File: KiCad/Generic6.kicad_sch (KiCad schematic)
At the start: 19 parts, among them J1 Shelly, J2 SPOX, J3 Conn_01x05, U1 ESP32-PICO-MINI-02, U2 LMR16006+FB

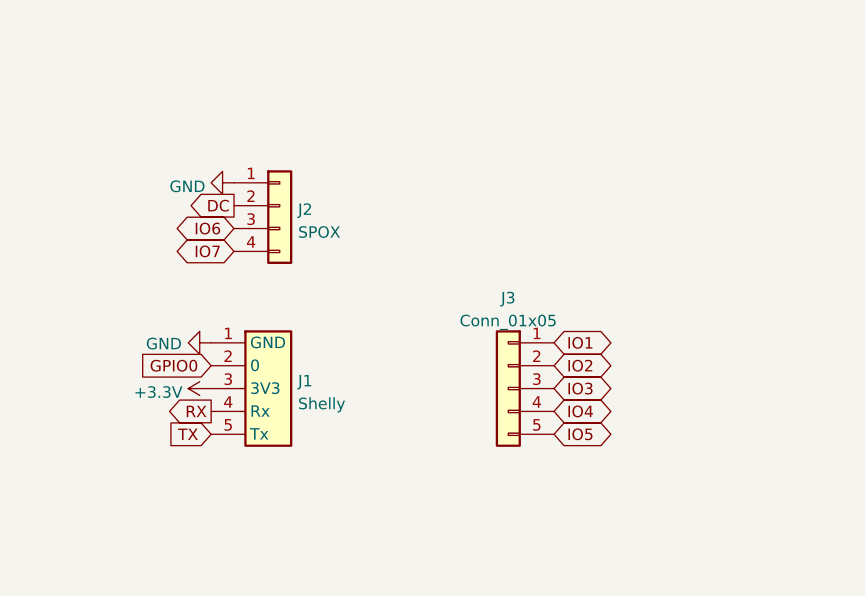
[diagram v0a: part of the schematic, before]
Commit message: Tidy Generic 4 Started on Generic 6
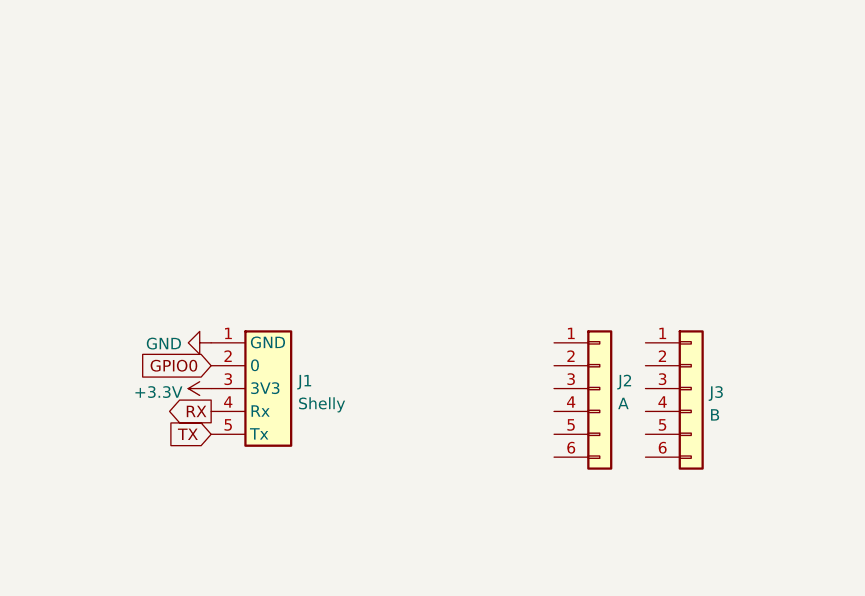
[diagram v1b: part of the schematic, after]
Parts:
- removed J2: SPOX, RevK:Molex_MiniSPOX_H4RA, symbol Connector_Generic:Conn_01x04
- removed J3: Conn_01x05, Connector_PinSocket_2.54mm:PinSocket_1x05_P2.54mm_Vertical, symbol Connector_Generic:Conn_01x05
- added J2: A, Connector_PinHeader_2.54mm:PinHeader_1x05_P2.54mm_Vertical, symbol Connector_Generic:Conn_01x06
- added J3: B, Connector_PinHeader_2.54mm:PinHeader_1x05_P2.54mm_Vertical, symbol Connector_Generic:Conn_01x06
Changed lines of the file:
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@@
     (stroke (width 0) (type default) (color 0 0 0 0))
-  )
-  (global_label "IO4" (shape bidirectional) (at 177.8 106.68 0) (fields_autoplaced)
-    (effects (font (size 1.27 1.27)) (justify left))
-    (property "Intersheet References" "${INTERSHEET_REFS}" (id 0) (at 183.269 106.7594 0)
-      (effects (font (size 1.27 1.27)) (justify left) hide)
-    )
   )
   (global_label "DC" (shape input) (at 136.525 36.83 180) (fields_autoplaced)
@@
     )
   )
-  (global_label "IO2" (shape bidirectional) (at 177.8 101.6 0) (fields_autoplaced)
-    (effects (font (size 1.27 1.27)) (justify left))
-    (property "Intersheet References" "${INTERSHEET_REFS}" (id 0) (at 183.269 101.6794 0)
-      (effects (font (size 1.27 1.27)) (justify left) hide)
-    )
-  )
   (global_label "IO4" (shape bidirectional) (at 50.8 83.82 180) (fields_autoplaced)
     (effects (font (size 1.27 1.27)) (justify right))
@@
     )
   )
-  (global_label "IO3" (shape bidirectional) (at 177.8 104.14 0) (fields_autoplaced)
-    (effects (font (size 1.27 1.27)) (justify left))
-    (property "Intersheet References" "${INTERSHEET_REFS}" (id 0) (at 183.269 104.2194 0)
-      (effects (font (size 1.27 1.27)) (justify left) hide)
-    )
-  )
   (global_label "R" (shape input) (at 81.28 71.12 0) (fields_autoplaced)
     (effects (font (size 1.27 1.27)) (justify left))
     (property "Intersheet References" "${INTERSHEET_REFS}" (id 0) (at 184.15 166.37 0)
       (effects (font (size 1.27 1.27)) hide)
-    )
-  )
-  (global_label "IO5" (shape bidirectional) (at 177.8 109.22 0) (fields_autoplaced)
-    (effects (font (size 1.27 1.27)) (justify left))
-    (property "Intersheet References" "${INTERSHEET_REFS}" (id 0) (at 183.269 109.1406 0)
-      (effects (font (size 1.27 1.27)) (justify left) hide)
     )
   )
@@
     )
   )
-  (global_label "IO7" (shape bidirectional) (at 142.24 88.9 180) (fields_autoplaced)
-    (effects (font (size 1.27 1.27)) (justify right))
-    (property "Intersheet References" "${INTERSHEET_REFS}" (id 0) (at 136.771 88.8206 0)
-      (effects (font (size 1.27 1.27)) (justify right) hide)
-    )
-  )
   (global_label "IO2" (shape bidirectional) (at 81.28 76.2 0) (fields_autoplaced)
     (effects (font (size 1.27 1.27)) (justify left))
@@
     )
   )
-  (global_label "IO6" (shape bidirectional) (at 142.24 86.36 180) (fields_autoplaced)
-    (effects (font (size 1.27 1.27)) (justify right))
-    (property "Intersheet References" "${INTERSHEET_REFS}" (id 0) (at 136.771 86.4394 0)
-      (effects (font (size 1.27 1.27)) (justify right) hide)
-    )
-  )
-  (global_label "DC" (shape output) (at 142.24 83.82 180) (fields_autoplaced)
-    (effects (font (size 1.27 1.27)) (justify right))
-    (property "Intersheet References" "${INTERSHEET_REFS}" (id 0) (at 137.3758 83.7406 0)
-      (effects (font (size 1.27 1.27)) (justify right) hide)
-    )
-  )
-  (global_label "IO1" (shape bidirectional) (at 177.8 99.06 0) (fields_autoplaced)
-    (effects (font (size 1.27 1.27)) (justify left))
-    (property "Intersheet References" "${INTERSHEET_REFS}" (id 0) (at 183.269 99.1394 0)
-      (effects (font (size 1.27 1.27)) (justify left) hide)
-    )
-  )
   (global_label "G" (shape input) (at 53.34 116.84 180) (fields_autoplaced)
     (effects (font (size 1.27 1.27)) (justify right))
@@
     (pin "2")
   )
-  (symbol (lib_id "power:GND") (at 142.24 81.28 270) (unit 1)
-    (in_bom yes) (on_board yes) (fields_autoplaced)
-    (property "Reference" "#PWR09" (id 0) (at 135.89 81.28 0)
-      (effects (font (size 1.27 1.27)) hide)
-    )
-    (property "Value" "GND" (id 1) (at 139.0651 81.7138 90)
-      (effects (font (size 1.27 1.27)) (justify right))
-    )
-    (property "Footprint" "" (id 2) (at 142.24 81.28 0)
-      (effects (font (size 1.27 1.27)) hide)
-    )
-    (property "Datasheet" "" (id 3) (at 142.24 81.28 0)
-      (effects (font (size 1.27 1.27)) hide)
-    )
-    (pin "1")
+  (symbol (lib_id "Connector_Generic:Conn_01x06") (at 193.04 104.14 0) (unit 1)
+    (in_bom yes) (on_board yes) (fields_autoplaced)
+    (property "Reference" "J3" (id 0) (at 195.072 104.5753 0)
+      (effects (font (size 1.27 1.27)) (justify left))
+    )
+    (property "Value" "B" (id 1) (at 195.072 107.1122 0)
+      (effects (font (size 1.27 1.27)) (justify left))
+    )
+    (property "Footprint" "Connector_PinHeader_2.54mm:PinHeader_1x05_P2.54mm_Vertical" (id 2) (at 193.04 104.14 0)
+      (effects (font (size 1.27 1.27)) hide)
+    )
+    (property "Datasheet" "~" (id 3) (at 193.04 104.14 0)
+      (effects (font (size 1.27 1.27)) hide)
+    )
+    (pin "1")
+    (pin "2")
+    (pin "3")
+    (pin "4")
+    (pin "5")
+    (pin "6")
   )
   (symbol (lib_id "Device:R") (at 64.77 27.94 270) (unit 1)
@@
   (symbol (lib_id "power:GND") (at 147.32 53.34 0) (unit 1)
     (in_bom yes) (on_board yes) (fields_autoplaced)
-    (property "Reference" "#PWR010" (id 0) (at 147.32 59.69 0)
+    (property "Reference" "#PWR09" (id 0) (at 147.32 59.69 0)
       (effects (font (size 1.27 1.27)) hide)
     )
@@
     )
     (pin "1")
-  )
-  (symbol (lib_id "Connector_Generic:Conn_01x05") (at 172.72 104.14 0) (mirror y) (unit 1)
-    (in_bom yes) (on_board yes) (fields_autoplaced)
-    (property "Reference" "J3" (id 0) (at 172.72 94.0902 0))
-    (property "Value" "Conn_01x05" (id 1) (at 172.72 96.6271 0))
-    (property "Footprint" "Connector_PinSocket_2.54mm:PinSocket_1x05_P2.54mm_Vertical" (id 2) (at 172.72 104.14 0)
-      (effects (font (size 1.27 1.27)) hide)
-    )
-    (property "Datasheet" "~" (id 3) (at 172.72 104.14 0)
-      (effects (font (size 1.27 1.27)) hide)
-    )
-    (pin "1")
-    (pin "2")
-    (pin "3")
-    (pin "4")
-    (pin "5")
   )
   (symbol (lib_id "RevK:Shelly") (at 144.78 104.14 0) (unit 1)
@@
     (pin "1")
   )
+  (symbol (lib_id "Connector_Generic:Conn_01x06") (at 182.88 104.14 0) (unit 1)
+    (in_bom yes) (on_board yes) (fields_autoplaced)
+    (property "Reference" "J2" (id 0) (at 184.912 103.3053 0)
+      (effects (font (size 1.27 1.27)) (justify left))
+    )
+    (property "Value" "A" (id 1) (at 184.912 105.8422 0)
+      (effects (font (size 1.27 1.27)) (justify left))
+    )
+    (property "Footprint" "Connector_PinHeader_2.54mm:PinHeader_1x05_P2.54mm_Vertical" (id 2) (at 182.88 104.14 0)
+      (effects (font (size 1.27 1.27)) hide)
+    )
+    (property "Datasheet" "~" (id 3) (at 182.88 104.14 0)
+      (effects (font (size 1.27 1.27)) hide)
+    )
+    (pin "1")
+    (pin "2")
+    (pin "3")
+    (pin "4")
+    (pin "5")
+    (pin "6")
+  )
   (symbol (lib_id "Device:C") (at 39.37 27.94 90) (unit 1)
     (in_bom yes) (on_board yes) (fields_autoplaced)
@@
     (pin "2")
   )
-  (symbol (lib_id "Connector_Generic:Conn_01x04") (at 147.32 83.82 0) (unit 1)
-    (in_bom yes) (on_board yes) (fields_autoplaced)
-    (property "Reference" "J2" (id 0) (at 149.352 84.2553 0)
-      (effects (font (size 1.27 1.27)) (justify left))
-    )
-    (property "Value" "SPOX" (id 1) (at 149.352 86.7922 0)
-      (effects (font (size 1.27 1.27)) (justify left))
-    )
-    (property "Footprint" "RevK:Molex_MiniSPOX_H4RA" (id 2) (at 148.59 91.44 0)
-      (effects (font (size 1.27 1.27)) hide)
-    )
-    (property "Datasheet" "~" (id 3) (at 147.32 83.82 0)
-      (effects (font (size 1.27 1.27)) hide)
-    )
-    (pin "1")
-    (pin "2")
-    (pin "3")
-    (pin "4")
-  )
   (symbol (lib_id "power:+3.3V") (at 200.66 38.1 0) (unit 1)
     (in_bom yes) (on_board yes) (fields_autoplaced)
-    (property "Reference" "#PWR011" (id 0) (at 200.66 41.91 0)
+    (property "Reference" "#PWR010" (id 0) (at 200.66 41.91 0)
       (effects (font (size 1.27 1.27)) hide)
     )
@@
   (symbol (lib_id "power:GND") (at 200.66 45.72 0) (unit 1)
     (in_bom yes) (on_board yes) (fields_autoplaced)
-    (property "Reference" "#PWR012" (id 0) (at 200.66 52.07 0)
+    (property "Reference" "#PWR011" (id 0) (at 200.66 52.07 0)
       (effects (font (size 1.27 1.27)) hide)
     )
@@
       (reference "#PWR08") (unit 1) (value "+3.3V") (footprint "")
     )
-    (path "/1e8ea742-99a3-47cc-bbc1-ed8989b74db8"
+    (path "/43ac1e5e-55b4-4274-a7ec-fd3947e95aec"
       (reference "#PWR09") (unit 1) (value "GND") (footprint "")
     )
-    (path "/43ac1e5e-55b4-4274-a7ec-fd3947e95aec"
-      (reference "#PWR010") (unit 1) (value "GND") (footprint "")
-    )
     (path "/b8f1f158-9ded-4572-b813-5295c6b7e555"
-      (reference "#PWR011") (unit 1) (value "+3.3V") (footprint "")
+      (reference "#PWR010") (unit 1) (value "+3.3V") (footprint "")
     )
     (path "/f7a2cf2e-033d-4a1a-9ac8-18e3c1c37533"
-      (reference "#PWR012") (unit 1) (value "GND") (footprint "")
+      (reference "#PWR011") (unit 1) (value "GND") (footprint "")
     )
     (path "/aea0762f-9b4b-49c8-b311-2b433e5a47c4"
@@
       (reference "J1") (unit 1) (value "Shelly") (footprint "RevK:Shelly")
     )
-    (path "/af073fa6-a783-40f2-9751-692984a62ffc"
-      (reference "J2") (unit 1) (value "SPOX") (footprint "RevK:Molex_MiniSPOX_H4RA")
-    )
-    (path "/5d1de36e-0591-465f-a55e-a456bc8d900f"
-      (reference "J3") (unit 1) (value "Conn_01x05") (footprint "Connector_PinSocket_2.54mm:PinSocket_1x05_P2.54mm_Vertical")
+    (path "/ab4e121c-071f-4432-a221-b67e64d6ff8d"
+      (reference "J2") (unit 1) (value "A") (footprint "Connector_PinHeader_2.54mm:PinHeader_1x05_P2.54mm_Vertical")
+    )
+    (path "/1c00a70d-616e-4b89-9535-f65d46a741bd"
+      (reference "J3") (unit 1) (value "B") (footprint "Connector_PinHeader_2.54mm:PinHeader_1x05_P2.54mm_Vertical")
     )
     (path "/00000000-0000-0000-0000-0000610fe01a"
